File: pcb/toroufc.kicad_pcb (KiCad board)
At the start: 2 copper layers, 70.5 x 87.5 mm, 39 parts, among them J1 HAT, J10 RPAD, J11 POT1-3, J12 POT4-6, J13 REN1, J14 REN2, J15 I2C, J16 Conn_01x04_Male, J2 RKR1-2, J3 RKR3-4, J4 LVR1-2, J5 MASTER-BIG1, J6 BIG2-3-4, J7 NPAD, J8 HPAD, J9 LPAD, U1 BluePill

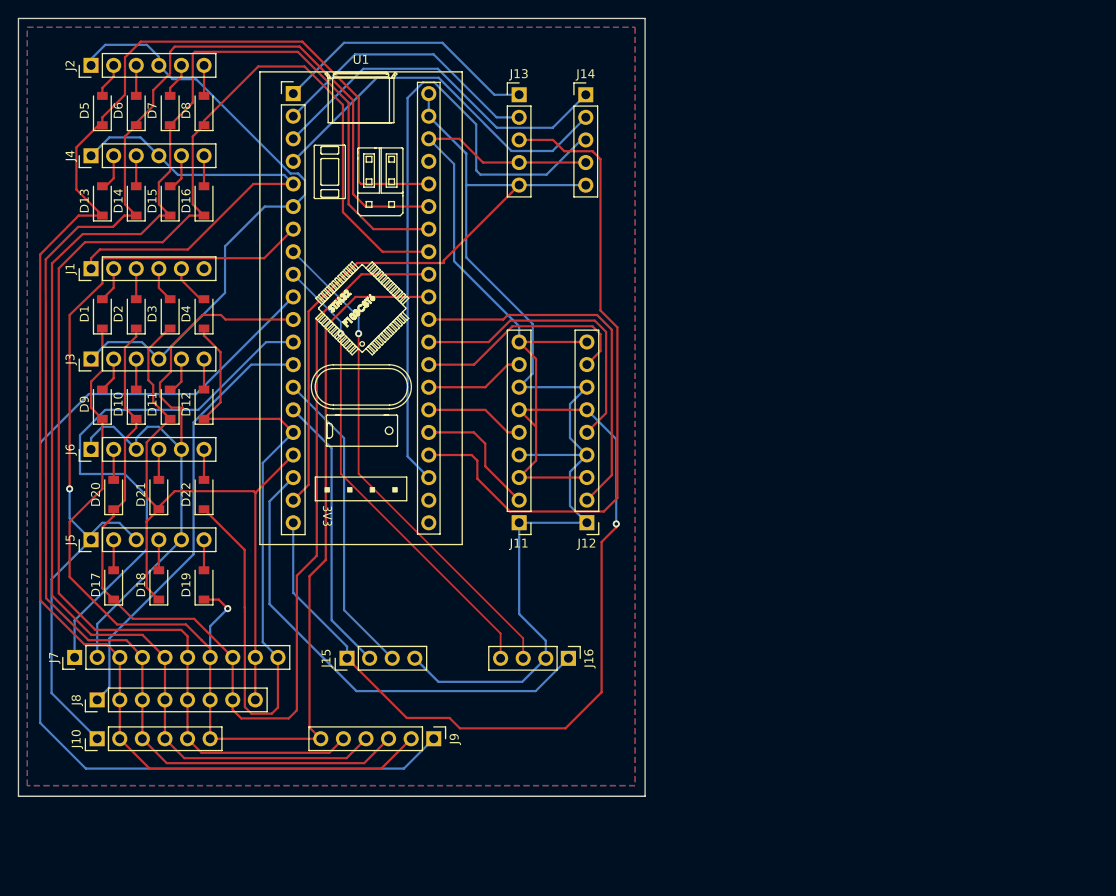
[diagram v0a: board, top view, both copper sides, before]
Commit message: Main PCB looking good.
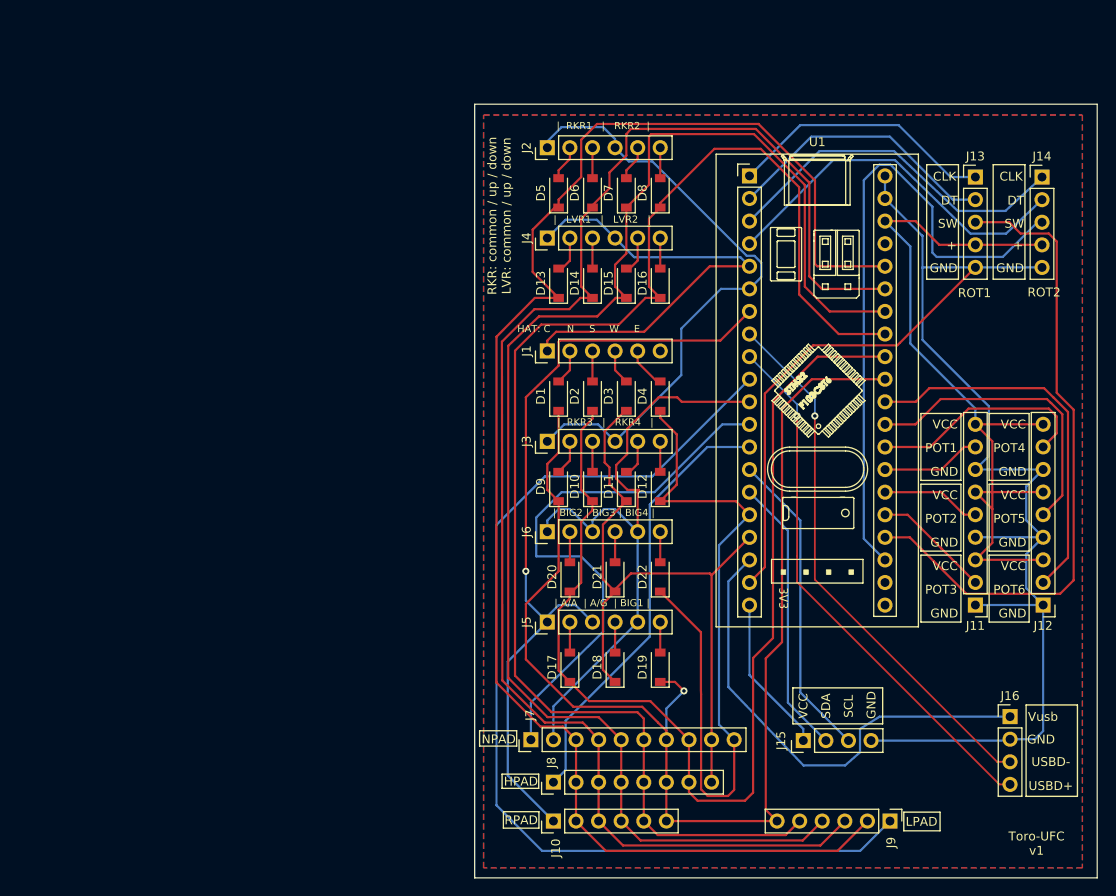
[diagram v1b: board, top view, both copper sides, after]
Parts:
- moved D10 52.1 mm to (122.5, 92.4)
- moved D14 52.1 mm to (122.5, 69.6)
- moved D2 52.1 mm to (122.5, 82.3)
- moved D6 52.1 mm to (122.5, 59.4)
- moved D1 52.1 mm to (118.7, 82.3)
- moved D11 52.1 mm to (126.4, 92.4)
- moved D12 52.1 mm to (130.2, 92.4)
- moved D13 52.1 mm to (118.7, 69.6)
- moved D15 52.1 mm to (126.4, 69.6)
- moved D16 52.1 mm to (130.2, 69.6)
- moved D17 52.1 mm to (120.0, 112.8)
- moved D18 52.1 mm to (125.1, 112.8)
- moved D19 52.1 mm to (130.2, 112.8)
- moved D20 52.1 mm to (120.0, 102.6)
- moved D21 52.1 mm to (125.1, 102.6)
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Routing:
- net VCC: track 173.3 -> 105.9 mm, vias 1 -> 0
- net /USBD+: track 52.8 -> 60.9 mm
- net /USBD-: track 56.4 -> 61.1 mm
- net /POT3: track 14.8 -> 13.3 mm
- net /REN1SW: track 74.6 -> 73.4 mm
- net /POT6: track 41.8 -> 42.6 mm
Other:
- board size 70.5 x 87.5 mm -> 70 x 87 mm
- board text added: "+"
- board text added: "CLK"
- board text added: "DT"
- board text added: "E"
- board text added: "GND"
- board text added: "HAT: C"
- board text added: "HPAD"
- board text added: "LPAD"
- board text added: "N"
- board text added: "NPAD"
- board text added: "POT1"
- board text added: "POT2"
- board text added: "POT3"
- board text added: "POT4"
- board text added: "POT5"
- board text added: "POT6"
- board text added: "RKR: common / up / down LVR: common / up / down"
- board text added: "ROT1"
- board text added: "ROT2"
- board text added: "RPAD"
- board text added: "S"
- board text added: "SCL"
- board text added: "SDA"
- board text added: "SW"
- board text added: "Toro-UFC v1"
- board text added: "USBD+"
- board text added: "USBD-"
- board text added: "VCC"
- board text added: "Vusb"
- board text added: "W"
- board text added: "| A/A | A/G | BIG1 |"
- board text added: "| BIG2 | BIG3 | BIG4 |"
- board text added: "| LVR1 | LVR2 |"
- board text added: "| RKR1 | RKR2 |"
- board text added: "| RKR3 | RKR4 |"
